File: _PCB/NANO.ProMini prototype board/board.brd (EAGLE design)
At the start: 85.7 x 100.1 mm, 35 parts, among them T1_5MM 5mm, T2_5MM 5mm, T3_5MM 5mm

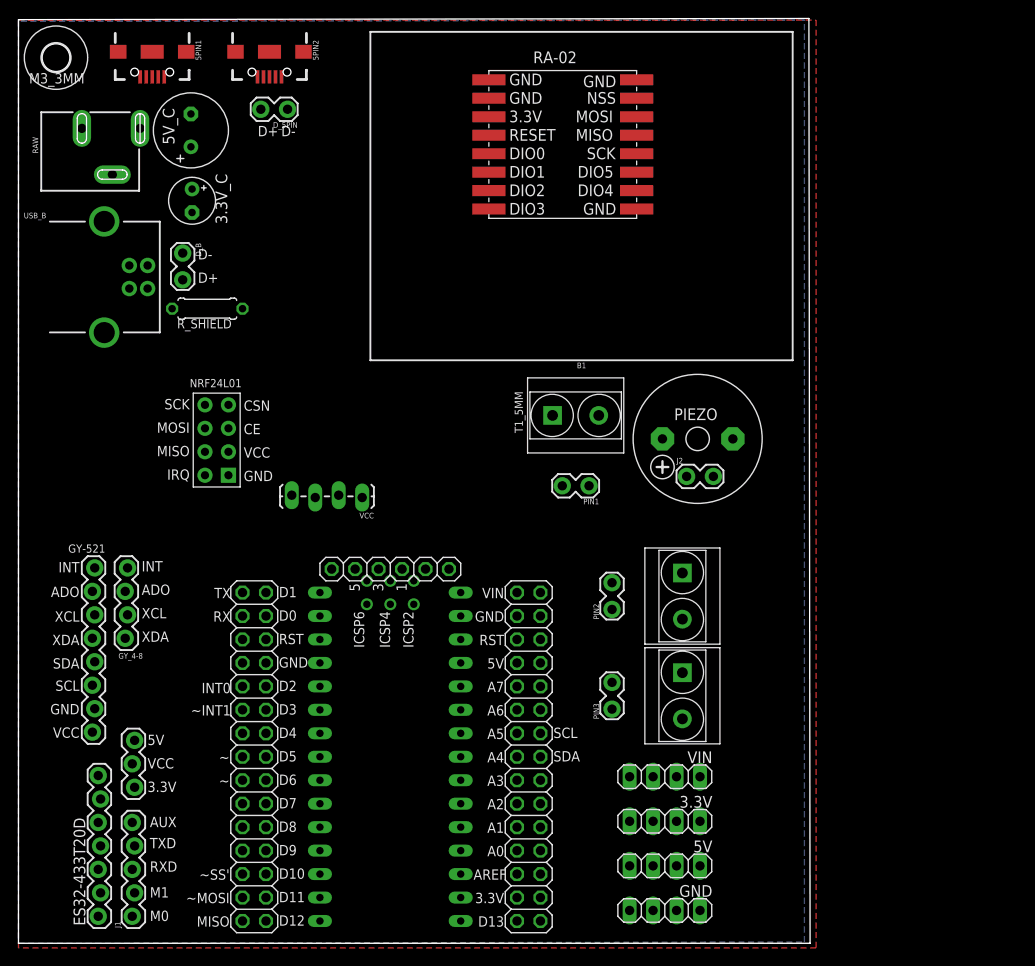
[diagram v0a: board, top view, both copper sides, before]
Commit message: update
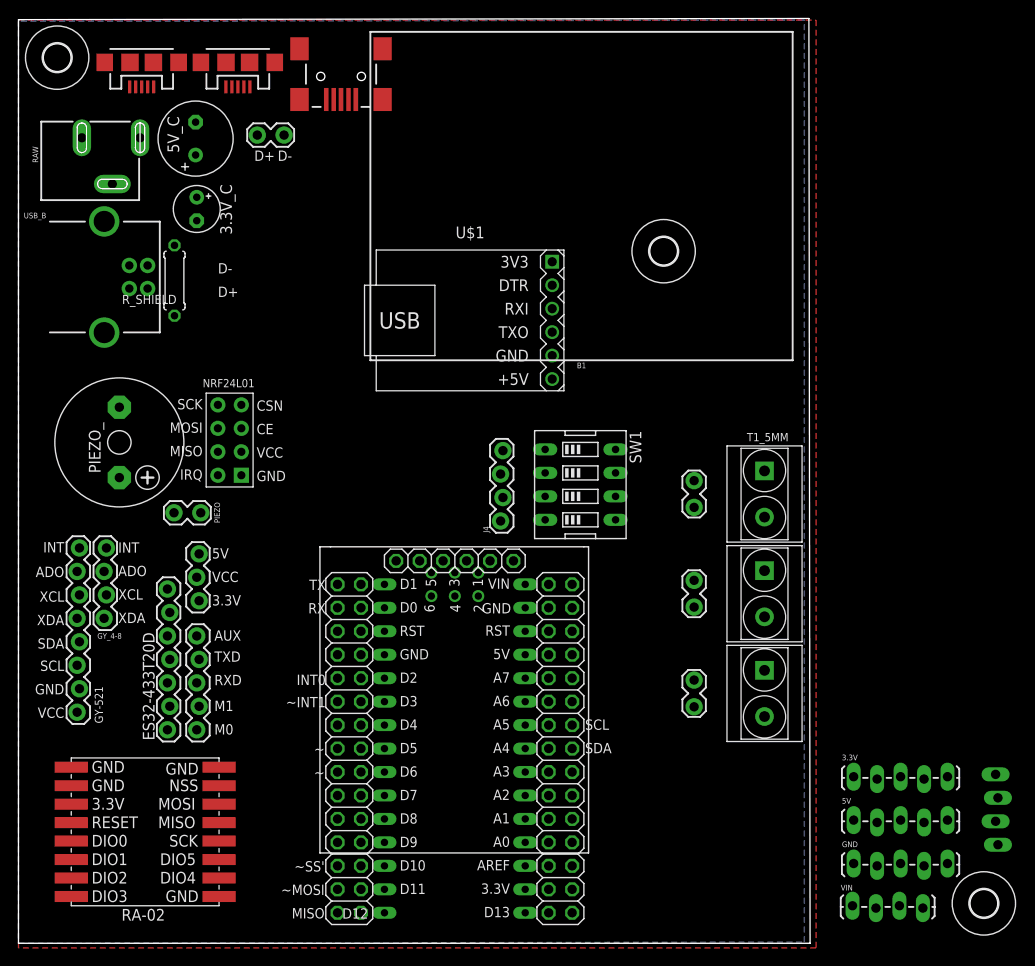
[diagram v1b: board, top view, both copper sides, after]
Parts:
- removed 5PIN1, 5PIN2: (no value), SparkFun-Connectors:USB-B-MICRO-SMD
- removed D_5PIN, D_B, J2: (no value), SparkFun-Connectors:1X02_LOCK
- removed VCC: (no value), SparkFun-Connectors:1X04_LOCK_LONGPADS
- added BOARD_POWER: (no value), SparkFun-Connectors:1X04_LOCK_LONGPADS
- added H2, H3: MOUNT-HOLE3.0, holes:3,0
- added J4: (no value), SparkFun-Connectors:1X04_LOCK
- added MICRO_1, MICRO_2: (no value), SparkFun-Connectors:USB-MICROB
- added MINI_1: USB_MINI-B_SMT, SparkFun-Connectors:USB-MINIB
- added PIEZO_: (no value), buzzer:F/CM12P
- added SW1: (no value), special:EDG-04
- added U$1: USB-SERIAL-CP2102, diy-modules:USB-SERIAL-CP2102
- added USB_DATA: (no value), SparkFun-Connectors:1X02_LOCK
- 3.3V, 5V, GND: device pinhead:1X04 -> SparkFun-Connectors:1X05_LOCK_LONGPADS
- PIEZO: device buzzer:F/CM12P -> SparkFun-Connectors:1X02_LOCK
- VIN: device pinhead:1X04 -> SparkFun-Connectors:1X04_LOCK_LONGPADS
- moved RA-02 87.1 mm to (13.7, 12.1)
- moved PIEZO 54.6 mm to (19.6, 46.6)
- moved VIN 24.7 mm to (90.3, 4.06), turned to 0 degrees
- moved T1_5MM 22.1 mm to (80.8, 48.6), turned to 0 degrees
- moved ES32-433T20D 21.5 mm to (16.3, 23.1)
- moved 3.3/5 21.4 mm to (19.4, 42.2)
- moved J1 21.4 mm to (19.4, 23.1)
- moved GND 21.1 mm to (90.4, 8.64), turned to 0 degrees
- moved 5V 21.0 mm to (90.4, 13.3), turned to 0 degrees
- moved 3.3V 21.0 mm to (90.4, 18.0), turned to 0 degrees
- moved PIN1 11.8 mm to (73.2, 47.4), turned to 90 degrees
- moved PH2 10.3 mm to (35.8, 21.1)
- moved PIN2 8.89 mm to (73.2, 36.6)
- moved PIN3 8.89 mm to (73.2, 25.8)
- moved T2_5MM 8.89 mm to (80.8, 37.8)
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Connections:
- removed net GND.3: RA-02.9
- removed net GND.4: RA-02.16
- removed net N$36: D_B.2, USB_B.D+
- removed net N$37: NANO.5V, PH1.23, PH1.24, VCC.3
- new net +5V: U$1.6
- new net 3V3: U$1.1
- new net N$38: BOARD_POWER.3, NANO.5V, PH1.23, PH1.24, SW1.5, SW1.6, SW1.7, SW1.8
- new net N$39: J4.1, SW1.4
- new net N$40: J4.2, SW1.3
- new net N$41: J4.3, SW1.2
- new net N$42: J4.4, SW1.1
- net 3.3V: now also 3.3V.5, BOARD_POWER.2; no longer 3.3V.1, VCC.2
- net 5V: now also 5V.5, BOARD_POWER.4, MICRO_1.VBUS, MICRO_2.VBUS, MINI_1.VBUS; no longer 5PIN1.VBUS, 5PIN2.VBUS, VCC.4
- net D+_5PIN: now also MICRO_1.D+, MICRO_2.D+, MINI_1.D+, USB_B.D+, USB_DATA.2; no longer 5PIN1.D+, 5PIN2.D+, D_5PIN.2
- net D-_5PIN: now also MICRO_1.D-, MICRO_2.D-, MINI_1.D-, USB_B.D-, USB_DATA.1; no longer 5PIN1.D-, 5PIN2.D-, D_5PIN.1
- net GND: now also MICRO_1.GND, MICRO_2.GND, MINI_1.GND, PIEZO_.-, U$1.5; no longer 5PIN1.GND, 5PIN2.GND, GND.1, GND.2, GND.3, GND.4, PIEZO.-
- net N$1: now also RA-02.16, RA-02.9
- net N$34: now also PIEZO.1, PIEZO.2, PIEZO_.+; no longer J2.1, J2.2, PIEZO.+
- net N$35: now also GND.1, GND.2, GND.3, GND.4, GND.5; no longer D_B.1, USB_B.D-
- net SHIELD_IN: now also MICRO_1.MT1, MICRO_1.MT2, MICRO_1.P$1, MICRO_1.P$2, MICRO_2.MT1, MICRO_2.MT2, MICRO_2.P$1, MICRO_2.P$2, MINI_1.S1, MINI_1.S2, MINI_1.S3, MINI_1.S4; no longer 5PIN1.SHIELD1, 5PIN1.SHIELD2, 5PIN1.SHIELD3, 5PIN2.SHIELD1, 5PIN2.SHIELD2, 5PIN2.SHIELD3
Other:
- board text added: "2"
- board text added: "4"
- board text added: "6"
- board text removed: "ICSP2"
- board text removed: "ICSP4"
- board text removed: "ICSP6"
- board text removed: "M3_3MM"
